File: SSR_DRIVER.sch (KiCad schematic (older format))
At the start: 7 parts, among them Q1 2N3904, U2 S102S01

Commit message: update,
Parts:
- D1: footprint (none) -> LED_SMD:LED_0805_2012Metric_Pad1.15x1.40mm_HandSolder
- R1, R2, R3, R4: footprint (none) -> Resistor_SMD:R_0805_2012Metric_Pad1.15x1.40mm_HandSolder
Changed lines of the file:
@@
 F 0 "R1" V 4304 3000 50  0000 C CNN
 F 1 "R331" V 4395 3000 50  0000 C CNN
-F 2 "" H 4500 3000 50  0001 C CNN
+F 2 "Resistor_SMD:R_0805_2012Metric_Pad1.15x1.40mm_HandSolder" H 4500 3000 50  0001 C CNN
 F 3 "~" H 4500 3000 50  0001 C CNN
 	1    4500 3000
@@
 F 0 "R2" H 4809 3446 50  0000 L CNN
 F 1 "R103" H 4809 3355 50  0000 L CNN
-F 2 "" H 4750 3400 50  0001 C CNN
+F 2 "Resistor_SMD:R_0805_2012Metric_Pad1.15x1.40mm_HandSolder" H 4750 3400 50  0001 C CNN
 F 3 "~" H 4750 3400 50  0001 C CNN
 	1    4750 3400
@@
 	5200 3650 5200 3200
 $Comp
-L power:GND #PWR0106
+L power:GND #PWR011
 U 1 1 5BCB4D36
 P 4950 3850
-F 0 "#PWR0106" H 4950 3600 50  0001 C CNN
+F 0 "#PWR011" H 4950 3600 50  0001 C CNN
 F 1 "GND" H 4955 3677 50  0000 C CNN
 F 2 "" H 4950 3850 50  0001 C CNN
@@
 F 0 "D1" V 4846 2132 50  0000 R CNN
 F 1 "LED_BLUE" V 4755 2132 50  0000 R CNN
-F 2 "" V 4800 2200 50  0001 C CNN
+F 2 "LED_SMD:LED_0805_2012Metric_Pad1.15x1.40mm_HandSolder" V 4800 2200 50  0001 C CNN
 F 3 "~" V 4800 2200 50  0001 C CNN
 	1    4800 2200
@@
 F 0 "R3" H 4859 2546 50  0000 L CNN
 F 1 "R331" H 4859 2455 50  0000 L CNN
-F 2 "" H 4800 2500 50  0001 C CNN
+F 2 "Resistor_SMD:R_0805_2012Metric_Pad1.15x1.40mm_HandSolder" H 4800 2500 50  0001 C CNN
 F 3 "~" H 4800 2500 50  0001 C CNN
 	1    4800 2500
@@
 F 0 "R4" H 5409 2346 50  0000 L CNN
 F 1 "R151" H 5409 2255 50  0000 L CNN
-F 2 "" H 5350 2300 50  0001 C CNN
+F 2 "Resistor_SMD:R_0805_2012Metric_Pad1.15x1.40mm_HandSolder" H 5350 2300 50  0001 C CNN
 F 3 "~" H 5350 2300 50  0001 C CNN
 	1    5350 2300
@@
 	6450 2500 7700 2500
 $Comp
-L power:VDD #PWR?
+L power:VDD #PWR012
 U 1 1 5BCBF013
 P 5050 1900
-F 0 "#PWR?" H 5050 1750 50  0001 C CNN
+F 0 "#PWR012" H 5050 1750 50  0001 C CNN
 F 1 "VDD" H 5067 2073 50  0000 C CNN
 F 2 "" H 5050 1900 50  0001 C CNN

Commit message: update,
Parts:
- removed Q1: 2N3904, Package_TO_SOT_THT:TO-92_Inline, symbol Transistor_BJT:2N3904
- added Q?: 2N3904(1AM), Package_TO_SOT_THT:TO-92_Inline, symbol taobao-transistor:2N3904(1AM)
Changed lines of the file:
@@
 $EndDescr
-$Comp
-L Transistor_BJT:2N3904 Q1
-U 1 1 5BCB4AD7
-P 5100 3000
-F 0 "Q1" H 5291 3046 50  0000 L CNN
-F 1 "2N3904" H 5291 2955 50  0000 L CNN
-F 2 "Package_TO_SOT_THT:TO-92_Inline" H 5300 2925 50  0001 L CIN
-F 3 "https://www.fairchildsemi.com/datasheets/2N/2N3904.pdf" H 5100 3000 50  0001 L CNN
-	1    5100 3000
-	1    0    0    -1
-$EndComp
 $Comp
 L taobao-r:R331 R1
@@
 	5050 2000 5350 2000
 Connection ~ 5050 2000
+$Comp
+L taobao-transistor:2N3904(1AM) Q?
+U 1 1 5BCBBF31
+P 5100 3000
+F 0 "Q?" H 5300 3050 50  0000 L CNN
+F 1 "2N3904(1AM)" H 5300 3000 50  0000 L CNN
+F 2 "Package_TO_SOT_THT:TO-92_Inline" H 5300 2925 50  0001 L CIN
+F 3 "" H 5100 3000 50  0001 L CNN
+	1    5100 3000
+	1    0    0    -1
+$EndComp
 $EndSCHEMATC

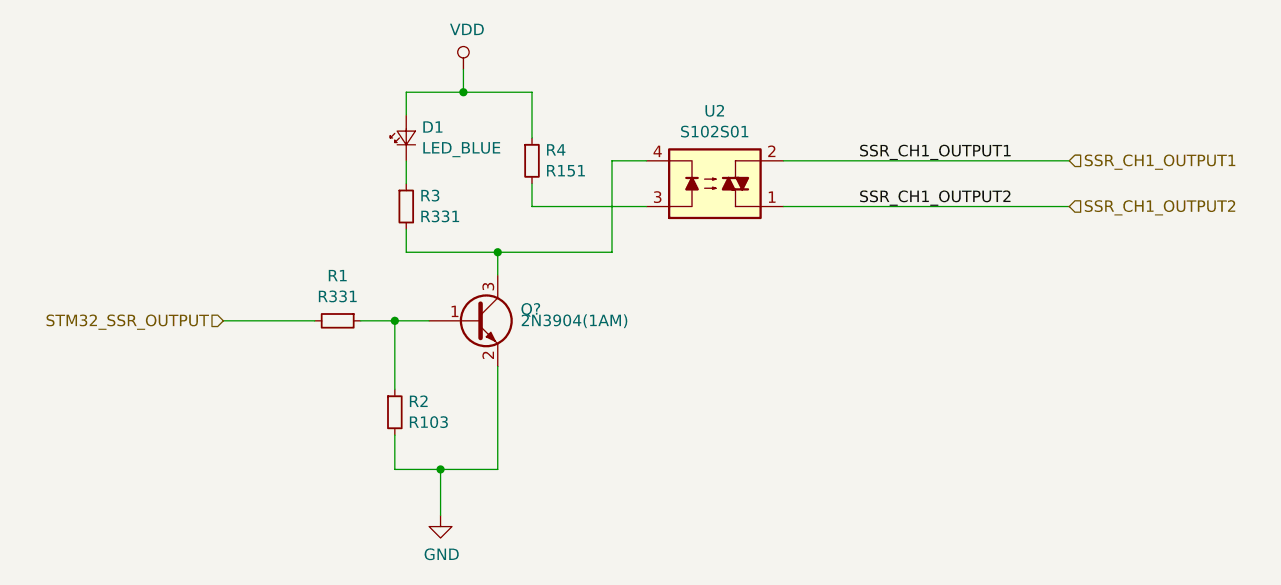
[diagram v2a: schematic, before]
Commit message: update,
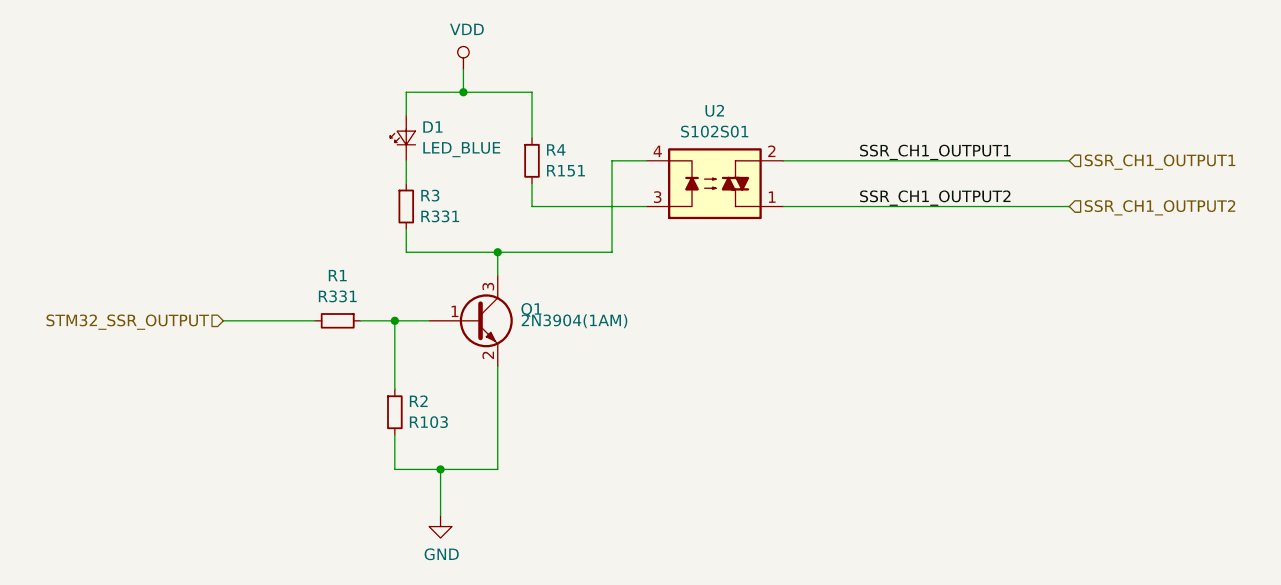
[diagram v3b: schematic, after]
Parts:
- Q1: renamed from Q?; footprint Package_TO_SOT_THT:TO-92_Inline -> Package_TO_SOT_SMD:SOT-23_Handsoldering
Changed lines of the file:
@@
 Connection ~ 5050 2000
 $Comp
-L taobao-transistor:2N3904(1AM) Q?
+L taobao-transistor:2N3904(1AM) Q1
 U 1 1 5BCBBF31
 P 5100 3000
-F 0 "Q?" H 5300 3050 50  0000 L CNN
+F 0 "Q1" H 5300 3050 50  0000 L CNN
 F 1 "2N3904(1AM)" H 5300 3000 50  0000 L CNN
-F 2 "Package_TO_SOT_THT:TO-92_Inline" H 5300 2925 50  0001 L CIN
+F 2 "Package_TO_SOT_SMD:SOT-23_Handsoldering" H 5300 2925 50  0001 L CIN
 F 3 "" H 5100 3000 50  0001 L CNN
 	1    5100 3000
